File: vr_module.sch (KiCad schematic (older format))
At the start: 34 parts, among them J1 Conn_01x07, U1 MAX9142, U2 NC7SB3157P6X, U3 74HC00, U4 NC7SB3157P6X, U5 SRV05-4, U6 MCP6004

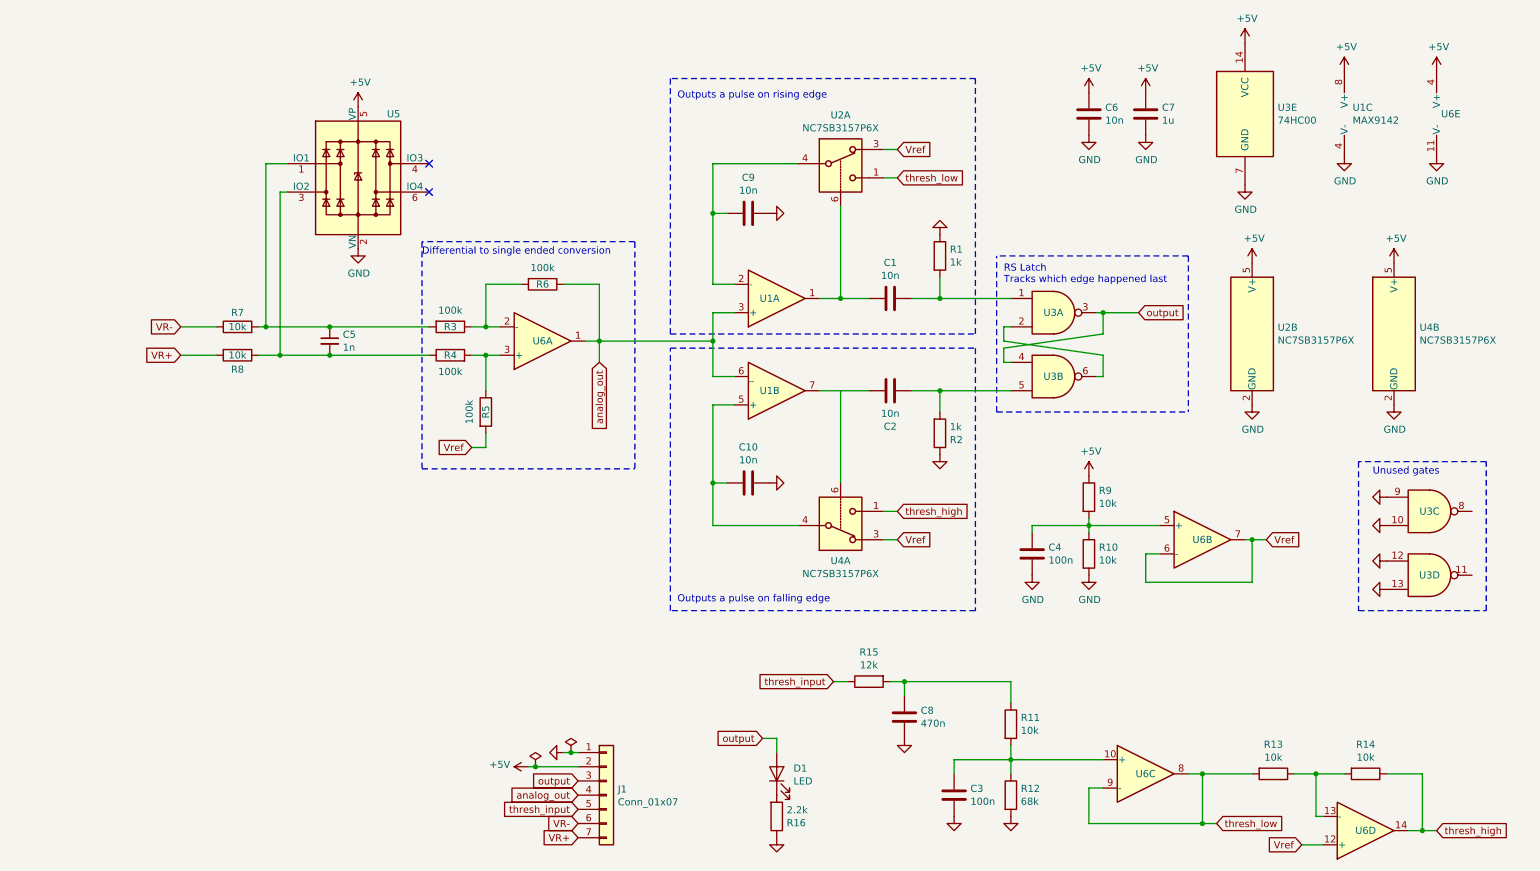
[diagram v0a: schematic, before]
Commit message: rev b improvements
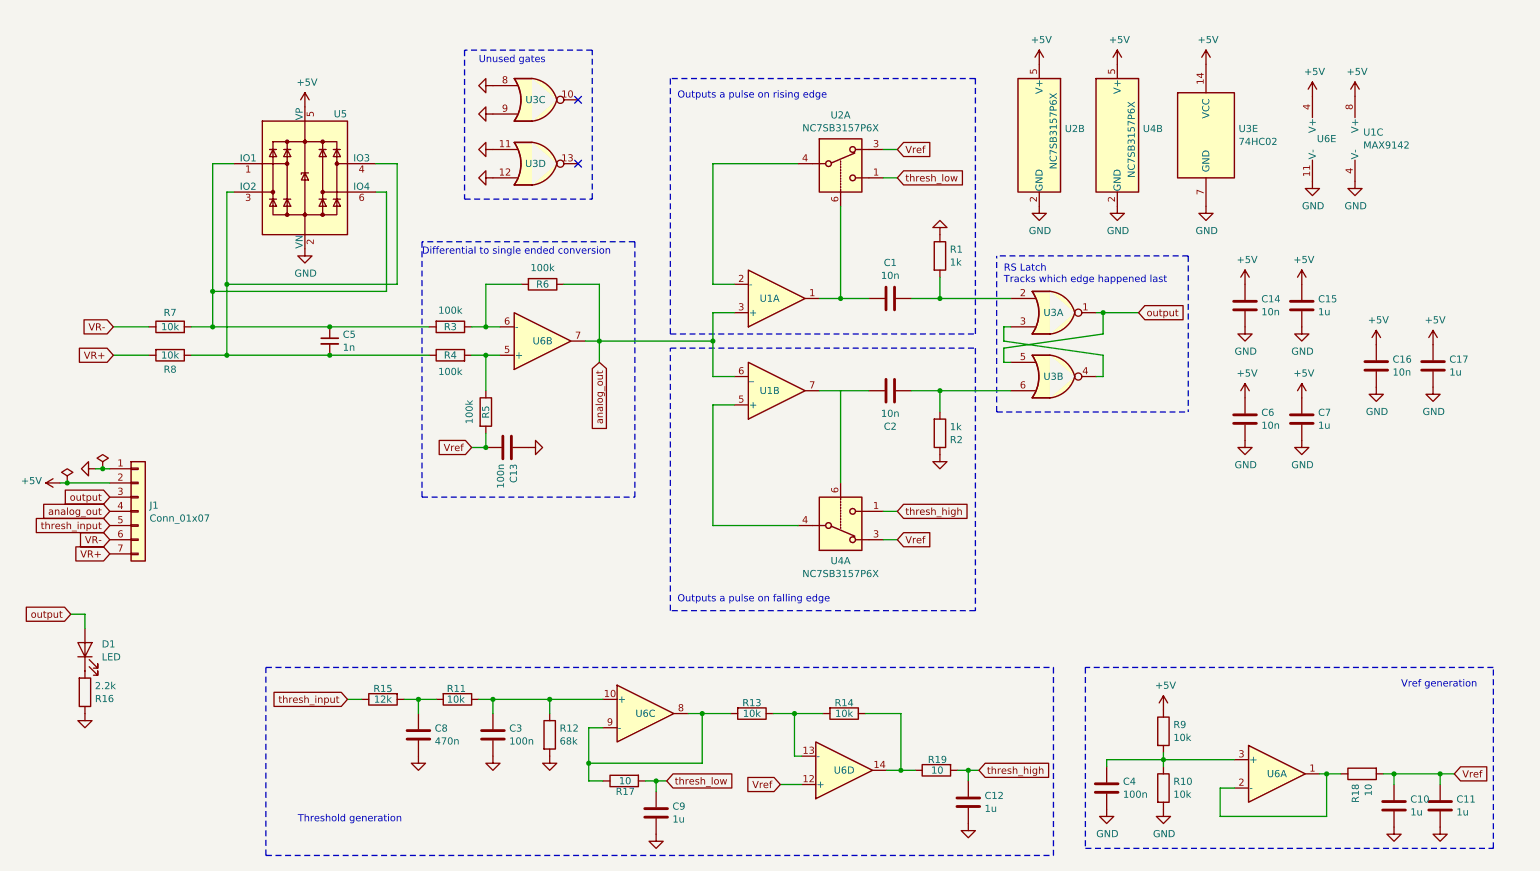
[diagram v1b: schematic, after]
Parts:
- removed U3: 74HC00, Package_SO:SOIC-14_3.9x8.7mm_P1.27mm, symbol 74xx:74HC00
- added C11, C12, C15, C17: 1u, Capacitor_SMD:C_0402_1005Metric, symbol Device:C
- added C13: 100n, Capacitor_SMD:C_0402_1005Metric, symbol Device:C
- added C14, C16: 10n, Capacitor_SMD:C_0402_1005Metric, symbol Device:C
- added R17, R18, R19: 10, Resistor_SMD:R_0402_1005Metric, symbol Device:R
- added U3: 74HC02, Package_SO:SOIC-14_3.9x8.7mm_P1.27mm, symbol 74xx:74HC02
- C10, C9: value 10n -> 1u; LCSC C15195 -> C52923
- C7: footprint Capacitor_SMD:C_0603_1608Metric -> Capacitor_SMD:C_0402_1005Metric; LCSC C15849 -> C52923
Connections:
- net +5V: now also C14.1, C15.1, C16.1, C17.1, U3.14 (VCC)
- net GND: now also C10.2, C9.2, C11.2, C12.2, C13.1, C14.2, C15.2, C16.2, C17.2, U3.11, U3.12, U3.7 (GND), U3.8, U3.9; no longer C10.1, C9.1
- net Vref: now also C10.1, C11.1, C13.2, R18.2; no longer U6.6 (-), U6.7
- net analog_out: now also U6.7; no longer U6.1
- net output: now also U3.1, U3.5
- net thresh_high: now also C12.1, R19.2; no longer R14.1, U6.14
- net thresh_low: now also C9.1, R17.2; no longer R13.2, U6.8, U6.9 (-)
- net at C1.1, R1.2: now also U3.2
- net at C2.1, R2.2: now also U3.6
- net at U1.2 (-), U2.4: no longer C9.2
- net at U1.5 (+), U4.4: no longer C10.2
- net at R3.1, R6.2: now also U6.6 (-); no longer U6.2 (-)
- net at R4.2, R5.1: now also U6.5 (+); no longer U6.3 (+)
- net at C4.1, R10.1, R9.2: now also U6.3 (+); no longer U6.5 (+)
- net at C3.1, R12.1, U6.10 (+): now also R11.1; no longer R11.2
- net at C5.1, R3.2, R7.2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: now also U5.6 (IO4)
- net at C5.2, R4.1, R8.1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: now also U5.4 (IO3)
- net at C8.1, R15.2: now also R11.2; no longer R11.1
- new net: R18.1, U6.1, U6.2 (-)
- new net: R13.2, R17.1, U6.8, U6.9 (-)
- new net: R14.1, R19.1, U6.14
- new net: U3.3, U3.4
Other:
- note added: "Threshold generation"
- note added: "Vref generation"
- moved on the sheet: C3, C4, C6, C7, C8, D1, J1, R10, R11, R12, R13, R14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
